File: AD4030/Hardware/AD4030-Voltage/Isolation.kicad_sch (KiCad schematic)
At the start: 26 parts, among them J401 Conn_01x08, J402 Conn_01x07, J403 PMOD, J404 PMOD, U401 ADuM260N1, U402 ADuM260N1

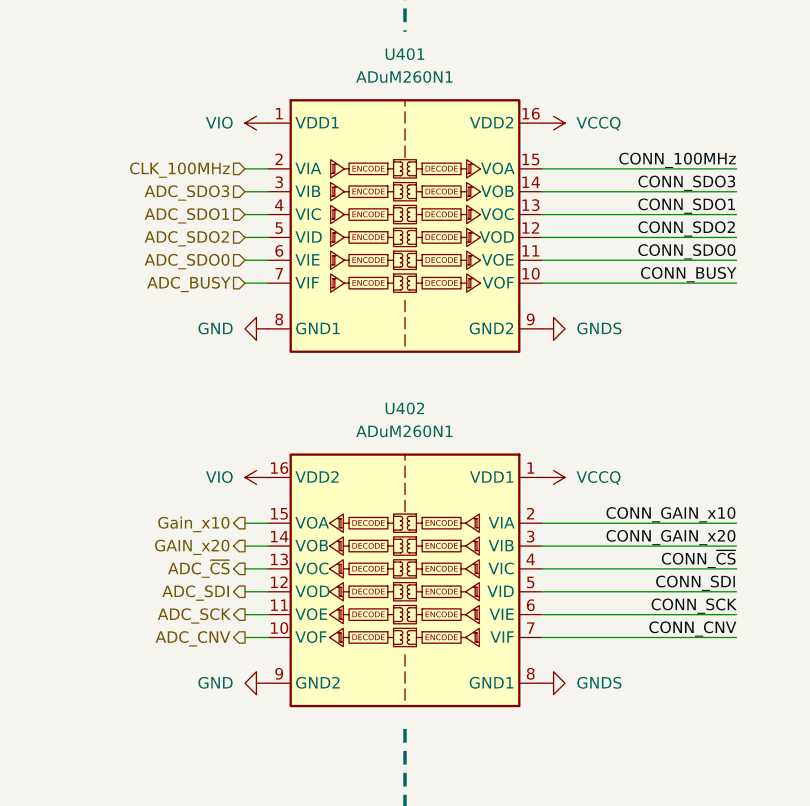
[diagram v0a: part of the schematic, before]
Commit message: Development
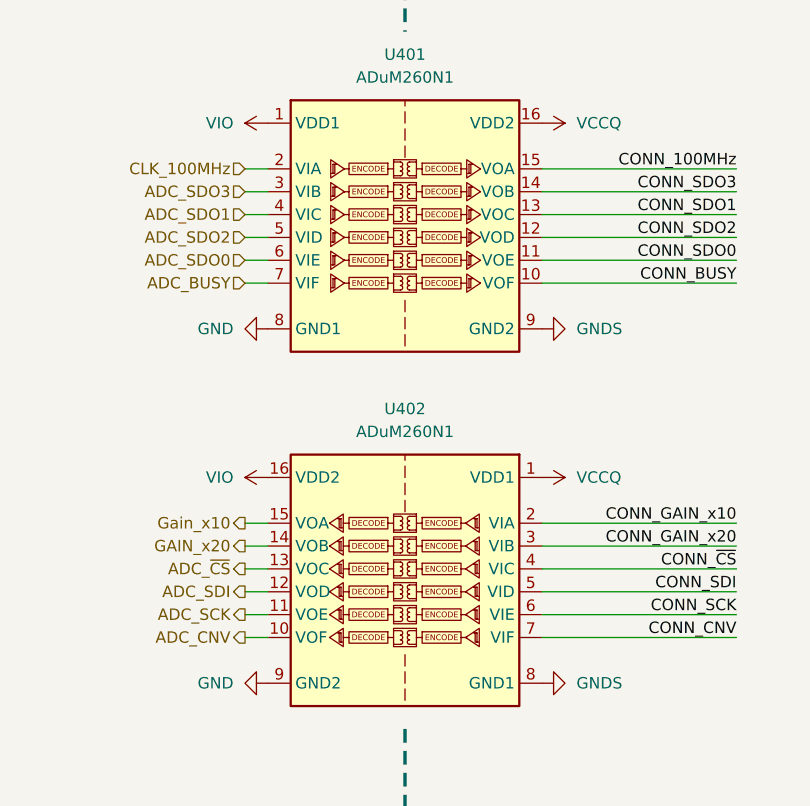
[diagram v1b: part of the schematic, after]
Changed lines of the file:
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@@
 (kicad_sch
-	(version 20231120)
+	(version 20250114)
 	(generator "eeschema")
-	(generator_version "8.0")
+	(generator_version "9.0")
 	(paper "A4")
 	(junction
@@
 	(label "CONN_GAIN_x10"
 		(at 148.59 115.57 0)
-		(fields_autoplaced yes)
 		(effects
 			(font
@@
 	(label "CONN_SDO1"
 		(at 195.58 66.04 0)
-		(fields_autoplaced yes)
 		(effects
 			(font
@@
 	(label "CONN_GAIN_x20"
 		(at 148.59 113.03 0)
-		(fields_autoplaced yes)
 		(effects
 			(font
@@
 	(label "CONN_BUSY"
 		(at 276.86 63.5 180)
-		(fields_autoplaced yes)
 		(effects
 			(font
@@
 	(label "CONN_~{CS}"
 		(at 148.59 110.49 0)
-		(fields_autoplaced yes)
 		(effects
 			(font
@@
 	(label "CONN_SDO0"
 		(at 195.58 63.5 0)
-		(fields_autoplaced yes)
 		(effects
 			(font
@@
 	(label "CONN_CNV"
 		(at 195.58 93.98 0)
-		(fields_autoplaced yes)
 		(effects
 			(font
@@
 	(label "CONN_GAIN_x20"
 		(at 138.43 105.41 180)
-		(fields_autoplaced yes)
 		(effects
 			(font
@@
 	(label "CONN_SDO1"
 		(at 138.43 68.58 180)
-		(fields_autoplaced yes)
 		(effects
 			(font
@@
 	(label "CONN_GAIN_x10"
 		(at 138.43 102.87 180)
-		(fields_autoplaced yes)
 		(effects
 			(font
@@
 	(label "CONN_SCK"
 		(at 148.59 78.74 0)
-		(fields_autoplaced yes)
 		(effects
 			(font
@@
 	(label "CONN_SDO3"
 		(at 148.59 63.5 0)
-		(fields_autoplaced yes)
 		(effects
 			(font
@@
 	(label "CONN_SDO2"
 		(at 148.59 68.58 0)
-		(fields_autoplaced yes)
 		(effects
 			(font
@@
 	(label "CONN_SDO3"
 		(at 138.43 66.04 180)
-		(fields_autoplaced yes)
 		(effects
 			(font
@@
 	(label "CONN_SDO0"
 		(at 148.59 71.12 0)
-		(fields_autoplaced yes)
 		(effects
 			(font
@@
 	(label "CONN_SDI"
 		(at 195.58 91.44 0)
-		(fields_autoplaced yes)
 		(effects
 			(font
@@
 	(label "CONN_SDO1"
 		(at 148.59 66.04 0)
-		(fields_autoplaced yes)
 		(effects
 			(font
@@
 	(label "CONN_100MHz"
 		(at 195.58 68.58 0)
-		(fields_autoplaced yes)
 		(effects
 			(font
@@
 	(label "CONN_SDO2"
 		(at 276.86 66.04 180)
-		(fields_autoplaced yes)
 		(effects
 			(font
@@
 	(label "CONN_SDO3"
 		(at 276.86 68.58 180)
-		(fields_autoplaced yes)
 		(effects
 			(font
@@
 	(label "CONN_CNV"
 		(at 148.59 76.2 0)
-		(fields_autoplaced yes)
 		(effects
 			(font
@@
 	(label "CONN_100MHz"
 		(at 148.59 60.96 0)
-		(fields_autoplaced yes)
 		(effects
 			(font
@@
 	(label "CONN_SDO0"
 		(at 138.43 73.66 180)
-		(fields_autoplaced yes)
 		(effects
 			(font
@@
 	(label "CONN_CNV"
 		(at 138.43 115.57 180)
-		(fields_autoplaced yes)
 		(effects
 			(font
@@
 	(label "CONN_SDI"
 		(at 138.43 110.49 180)
-		(fields_autoplaced yes)
 		(effects
 			(font
@@
 	(label "CONN_SCK"
 		(at 276.86 93.98 180)
-		(fields_autoplaced yes)
 		(effects
 			(font
@@
 	(label "CONN_~{CS}"
 		(at 276.86 91.44 180)
-		(fields_autoplaced yes)
 		(effects
 			(font
@@
 	(label "CONN_SDI"
 		(at 148.59 107.95 0)
-		(fields_autoplaced yes)
 		(effects
 			(font
@@
 	(label "CONN_SCK"
 		(at 138.43 113.03 180)
-		(fields_autoplaced yes)
 		(effects
 			(font
@@
 	(label "CONN_SDO2"
 		(at 138.43 71.12 180)
-		(fields_autoplaced yes)
 		(effects
 			(font
@@
 	(label "CONN_BUSY"
 		(at 138.43 76.2 180)
-		(fields_autoplaced yes)
 		(effects
 			(font
@@
 	(label "CONN_GAIN_x10"
 		(at 276.86 88.9 180)
-		(fields_autoplaced yes)
 		(effects
 			(font
@@
 	(label "CONN_BUSY"
 		(at 148.59 73.66 0)
-		(fields_autoplaced yes)
 		(effects
 			(font
@@
 	(label "CONN_100MHz"
 		(at 138.43 63.5 180)
-		(fields_autoplaced yes)
 		(effects
 			(font
@@
 	(label "CONN_GAIN_x20"
 		(at 195.58 88.9 0)
-		(fields_autoplaced yes)
 		(effects
 			(font
@@
 	(label "CONN_~{CS}"
 		(at 138.43 107.95 180)
-		(fields_autoplaced yes)
 		(effects
 			(font
@@
 		(shape output)
 		(at 83.82 105.41 180)
-		(fields_autoplaced yes)
 		(effects
 			(font
@@
 		(shape input)
 		(at 83.82 63.5 180)
-		(fields_autoplaced yes)
 		(effects
 			(font
@@
 		(shape input)
 		(at 83.82 73.66 180)
-		(fields_autoplaced yes)
 		(effects
 			(font
@@
 		(shape output)
 		(at 83.82 113.03 180)
-		(fields_autoplaced yes)
 		(effects
 			(font
@@
 		(shape output)
 		(at 83.82 102.87 180)
-		(fields_autoplaced yes)
 		(effects
 			(font
@@
 		(shape input)
 		(at 83.82 66.04 180)
-		(fields_autoplaced yes)
 		(effects
 			(font
@@
 		(shape input)
 		(at 83.82 68.58 180)
-		(fields_autoplaced yes)
 		(effects
 			(font
@@
 		(shape input)
 		(at 83.82 71.12 180)
-		(fields_autoplaced yes)
 		(effects
 			(font
@@
 		(shape output)
 		(at 83.82 107.95 180)
-		(fields_autoplaced yes)
 		(effects
 			(font
@@
 		(shape output)
 		(at 83.82 115.57 180)
-		(fields_autoplaced yes)
 		(effects
 			(font
@@
 		(shape output)
 		(at 83.82 110.49 180)
-		(fields_autoplaced yes)
 		(effects
 			(font
@@
 		(shape input)
 		(at 83.82 76.2 180)
-		(fields_autoplaced yes)
-		(effects
-			(font
+		(effects
+			(font
